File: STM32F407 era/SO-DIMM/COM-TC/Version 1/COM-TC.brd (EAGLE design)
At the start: 127 x 165.1 mm, 172 parts, among them J1 CON1, J2 CON1, J3 SO-DIMM-CPU, J4 FTDI_DEVICE, Q4 PMV20XNE, U1 IRF9332PBF, U10 SN65HVD232D, U11 MAX9926, U12 MCP6004-E/SL, U13 MCP6004-E/SL, U14 MCP6004-E/SL, U2 5V, U3 TPS54331D, U4 3,3V, U5 MAX9926, U6 MCP6004-E/SL, U7 LoPy, U8 GTL2000, X1 057-014-1

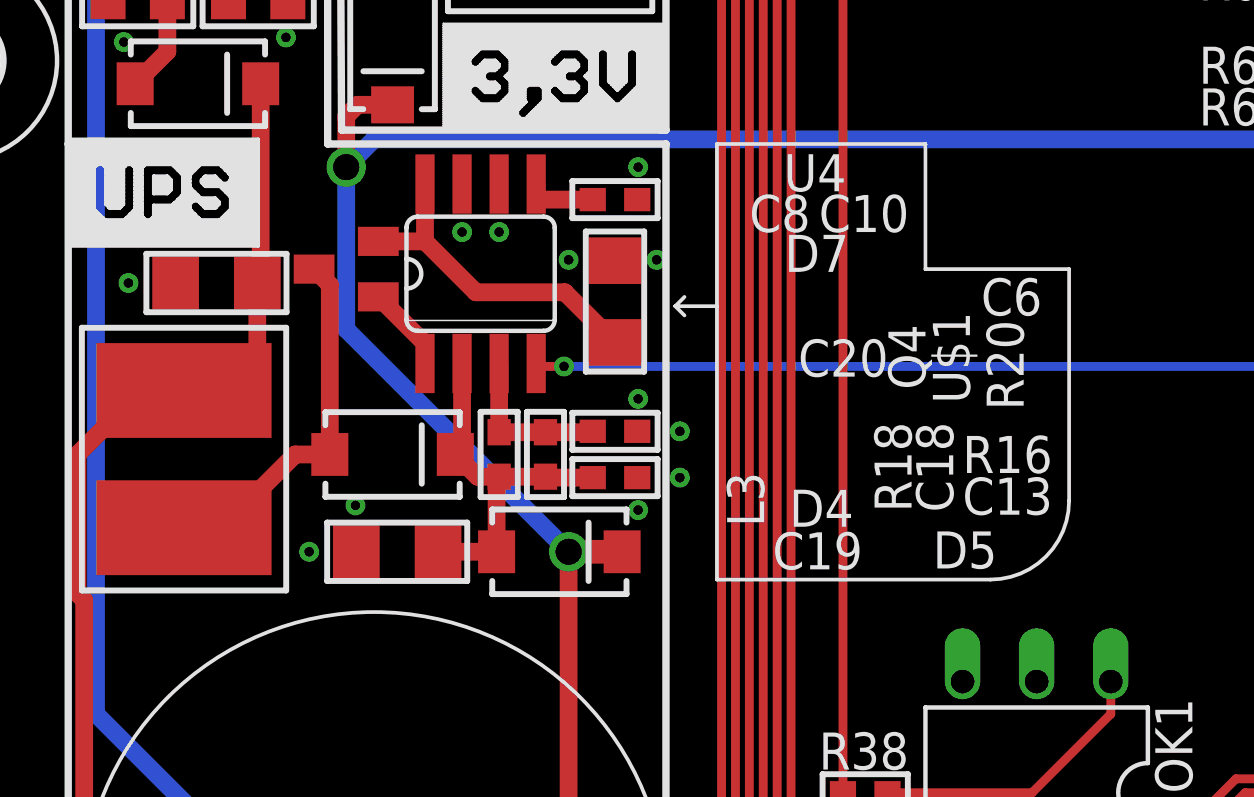
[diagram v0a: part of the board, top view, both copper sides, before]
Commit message: small error fixes
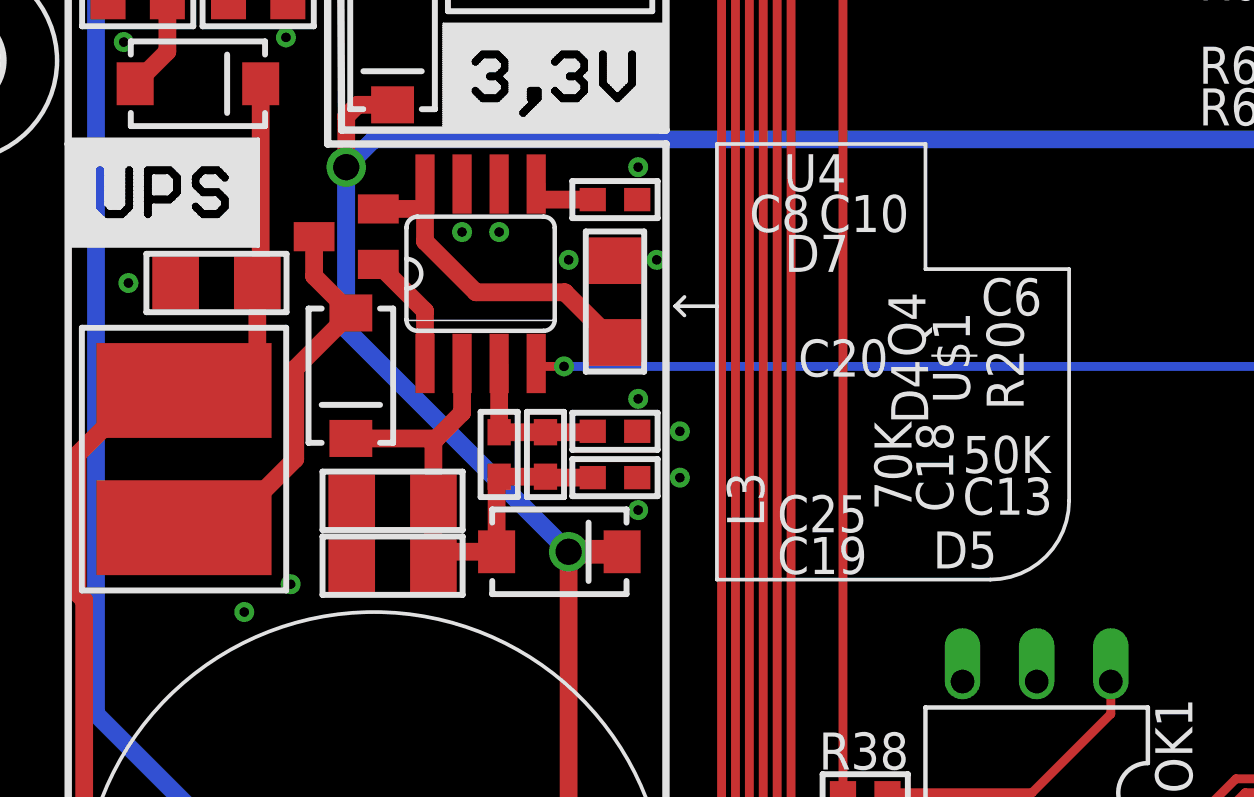
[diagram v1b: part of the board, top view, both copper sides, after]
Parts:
- added C25: 100u 6v3, microbuilder:1206
- C18: value 100n -> 47p
- C19: value 220u 6v3 -> 100u 6v3
- R20: value 10m -> 35m
- R69: value 3k24 -> 2k7
- moved D4 3.05 mm to (17.6, 76.2), turned to 270 degrees
- moved Q4 1.11 mm to (17.5, 81.0)
- moved C19 0.50 mm to (19.1, 69.7)
- renumbered R16 to 50K, R18 to 70K
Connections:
- net GND: now also C25.2
- net N$28: now also C25.1
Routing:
- net N$28: track 12.9 -> 18.5 mm
- net N$36: track 12.6 -> 15.0 mm
- net N$7: track 2.94 -> 4.06 mm
- net N$27: track 11.5 -> 12.4 mm

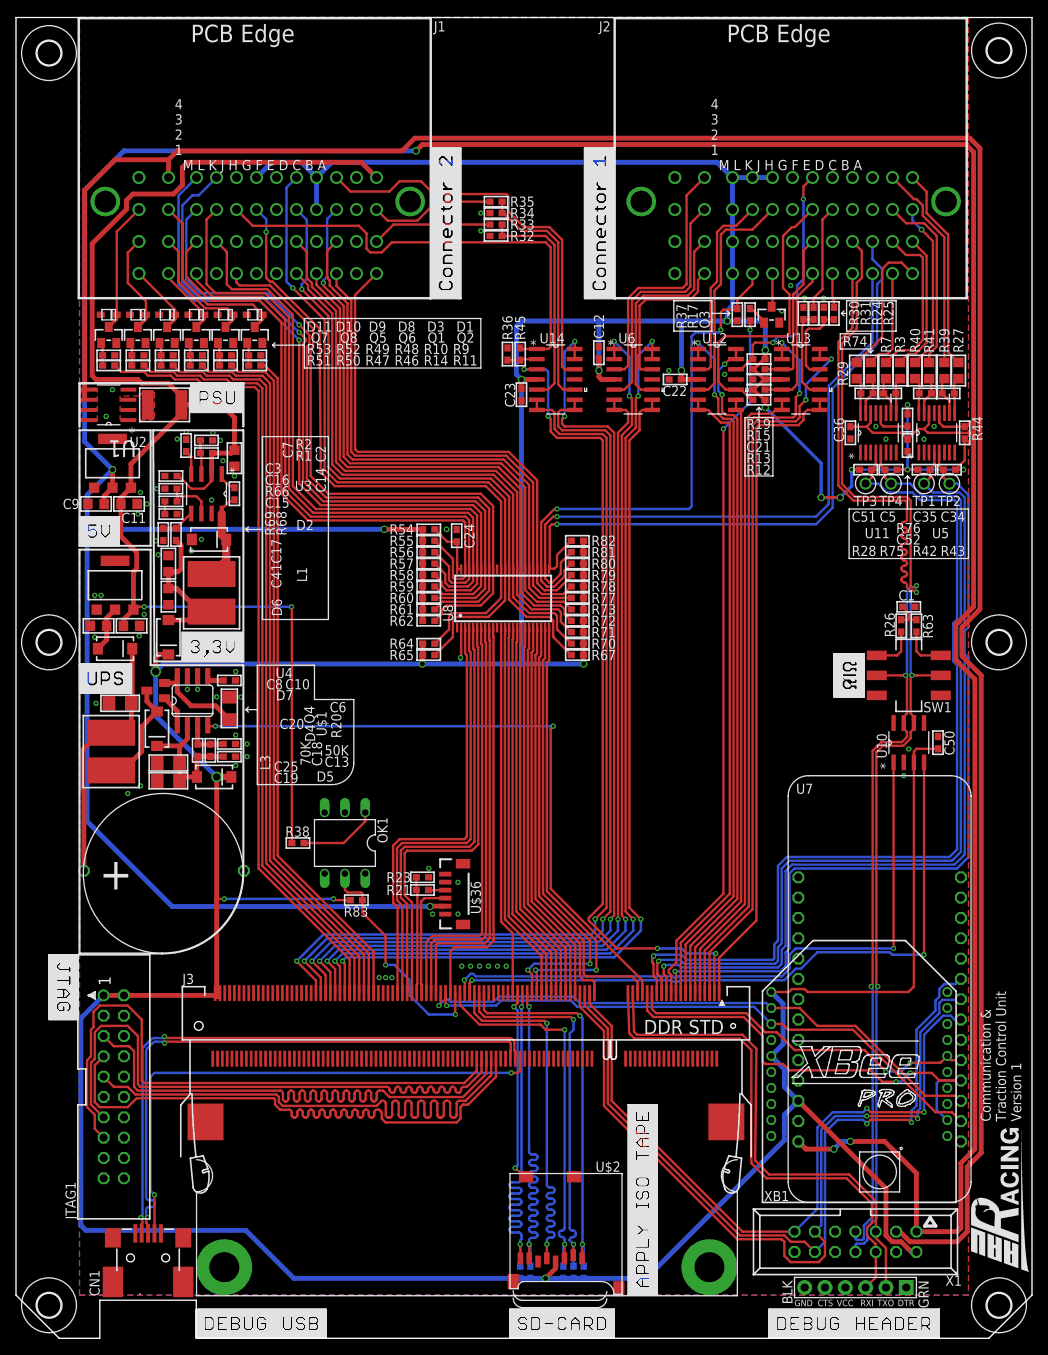
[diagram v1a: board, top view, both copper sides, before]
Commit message: error corrections
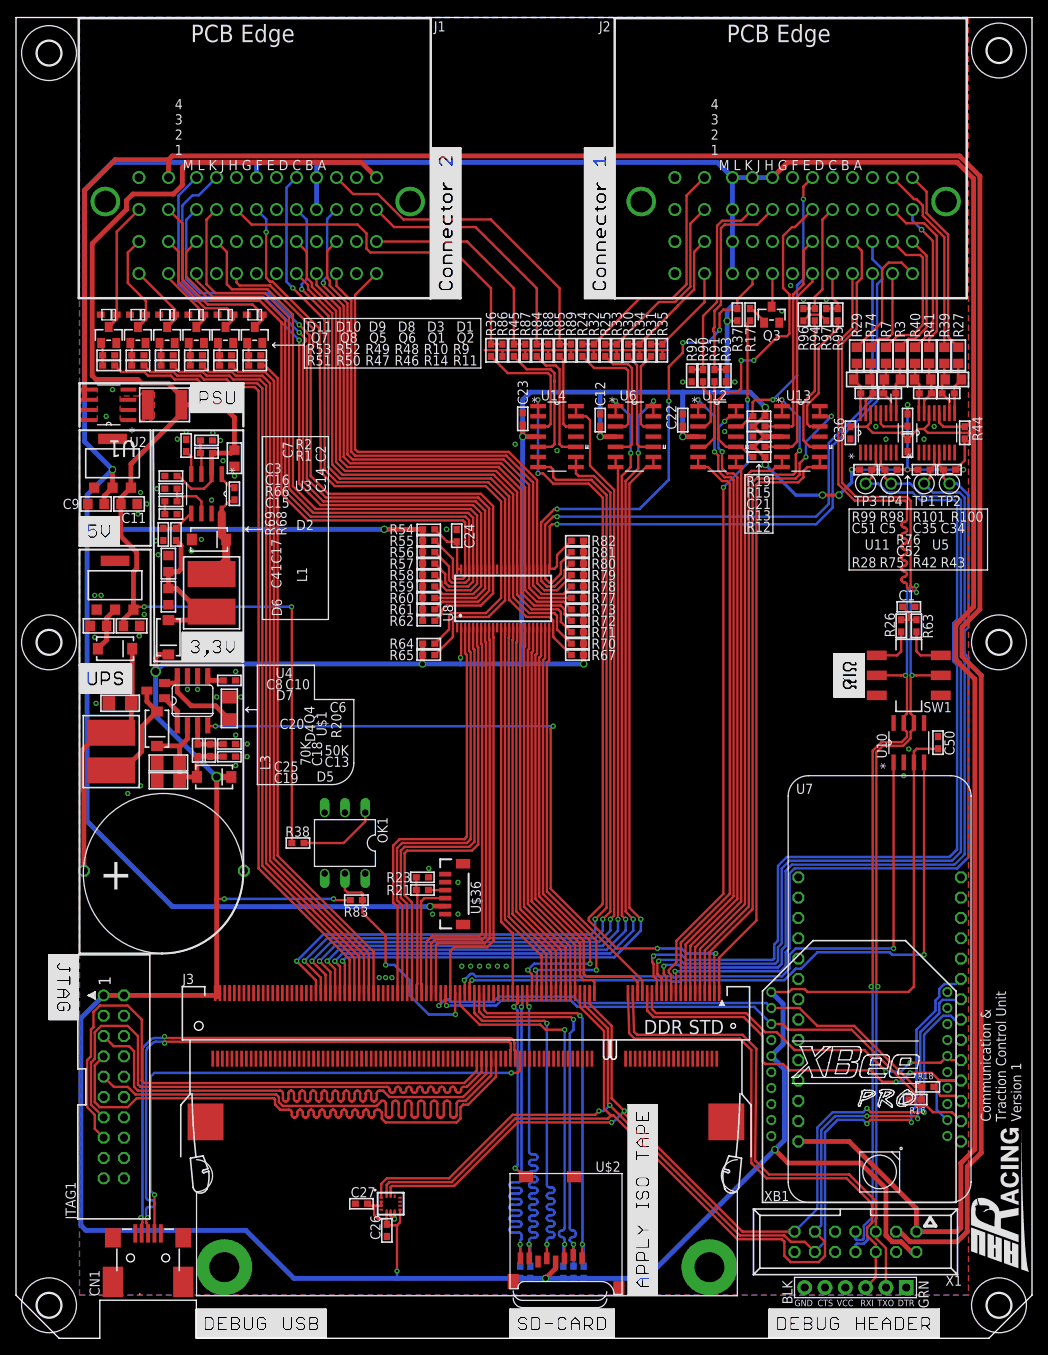
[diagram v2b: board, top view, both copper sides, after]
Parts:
- added C26, C27: 100n, microbuilder:_0603
- added R100, R101, R98, R99: 10k 0W5, microbuilder:_0805
- added R16, R86, R87, R88, R89, R92, R93, R96, R97: 976, microbuilder:_0603
- added R18, R84, R85, R90, R91, R94, R95: 499, microbuilder:_0603
- added U9: LSM6DS3, LSM6DS3:LGA14L_DOT_INDICATOR
- R24, R30, R36: value 976 -> 499
- R33, R35: value 499 -> 976
- moved R24 30.5 mm to (70.8, 123.5)
- moved R25 28.9 mm to (73.7, 123.5)
- moved R35 27.9 mm to (80.8, 123.5), turned to 270 degrees
- moved R34 24.8 mm to (77.9, 123.5), turned to 270 degrees
- moved R30 22.4 mm to (76.5, 123.5)
- moved R33 21.8 mm to (75.1, 123.5), turned to 270 degrees
- moved R31 20.8 mm to (79.4, 123.5)
- moved R32 18.8 mm to (72.2, 123.5), turned to 270 degrees
- moved C12 8.42 mm to (73.0, 114.8)
- moved U14 7.15 mm to (67.6, 112.7)
- moved U6 7.15 mm to (77.3, 112.7)
- moved R13 7.14 mm to (92.9, 111.4)
- moved C21 7.14 mm to (92.9, 112.7)
- moved R12 7.14 mm to (92.9, 110.2)
- moved R15 7.14 mm to (92.9, 114.0)
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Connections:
- removed net CURRENT1H: J2.E1, R25.1
- removed net CURRENT1L: R24.2, R25.2, U13.12
- removed net CURRENT2H: J2.E3, R31.1
- removed net CURRENT2L: R30.2, R31.2, U13.10
- removed net GSENSL: R32.2, R33.2, U14.5
- removed net VOUT: J3.3, U14.3
- removed net VOUTB: J1.H3, R45.2, U14.1
- removed net YAWL: R34.2, R35.2, U14.10
- new net CLUTCH-POT1: R31.2, U6.12
- new net CURRENT1: J2.E1, R95.1, R97.1
- new net CURRENT2: J2.E3, R94.1, R96.1
- new net GSENSL1: R25.2, U6.5
- new net GSENSL2: R91.2, U12.5
- new net GSENSL3: R95.2, U13.12
- new net N$34: R84.2, U14.10
- new net N$35: R18.2, U7.41
- new net N$38: R45.2, U14.5
- new net N$39: R36.2, U14.3
- new net STEERING-ANGLE: J1.H3, R36.1, R86.1
- new net STEERING-ANGLE1: R24.2, U6.3
- new net STEERING-ANGLE2: R90.2, U12.3
- new net STEERING-ANGLE3: R94.2, U13.10
- new net STEERING-ANGLEB: J3.3, U14.1, U14.2
- new net YAWL1: R30.2, U6.10
- net 3.3V: now also C26.1, C27.1, U9.2, U9.3, U9.5, U9.8; no longer J1.D3, J1.D4, J1.G4, J2.H4, J2.J4, J2.K1, J2.K2, J2.K3, J2.K4, U7.3,3V
- net 5.0V: now also J1.D3, J1.D4, J1.G4, J2.H4, J2.J4, J2.K1, J2.K2, J2.K3, J2.K4
- net CLUTCH-POT: now also R85.1, R89.1; no longer U14.12
- net GEARPOSAN: now also R91.1, R93.1; no longer U12.5
- net GND: now also C26.2, C27.2, R16.2, R32.2, R33.2, R34.2, R35.2, R86.2, R87.2, R88.2, R89.2, R92.2, R93.2, R96.2, R97.2, U9.12, U9.6, U9.7; no longer R24.1, R30.1, R32.1, R34.1, R36.1
- net GSENS: now also R45.1, R87.1; no longer R33.1
- net MISO: now also U9.1
- net MOSI: now also U9.14
- net N$11: now also R100.2
- net N$13: now also R85.2, U14.12; no longer R36.2, R45.1, U14.2
- net N$15: now also R101.1
- net N$16: now also R98.2
- net N$17: now also R101.2
- net N$18: now also R100.1
- net N$19: now also R99.1
- net N$25: now also R99.2
- net N$26: now also R98.1
- net SCK: now also U9.13
- net SPEED: now also R90.1, R92.1; no longer U12.3
- net TELE_RX: now also R16.1, R18.1; no longer U7.41
- net TRAVEL1: now also R25.1, R33.1; no longer U6.5
- net TRAVEL2: now also R24.1, R32.1; no longer U6.3
- net TRAVEL3: now also R30.1, R34.1; no longer U6.10
- net TRAVEL4: now also R31.1, R35.1; no longer U6.12
- net YAW: now also R84.1, R88.1; no longer R35.1
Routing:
- net VOUT: track 102.7 -> 0.00 mm, vias 4 -> 0
- net STEERING-ANGLEB: track 0.00 -> 96.8 mm, vias 0 -> 4
- net 3.3V: track 644.2 -> 560.6 mm, vias 20 -> 22
- net VOUTB: track 59.8 -> 0.00 mm
- net STEERING-ANGLE: track 0.00 -> 45.4 mm
- net GND: track 0.00 -> 34.7 mm, vias 62 -> 64
- net MISO: track 97.3 -> 131.7 mm, vias 2 -> 4
- net SCK: track 88.4 -> 122.7 mm, vias 2 -> 4
- net MOSI: track 100.4 -> 133.7 mm
- net YAWL: track 30.0 -> 0.00 mm
- net GSENSL: track 28.3 -> 0.00 mm
- net STEERING-ANGLE3: track 0.00 -> 17.9 mm
- net N$38: track 0.00 -> 17.2 mm
- net YAW: track 15.7 -> 32.5 mm
- net N$39: track 0.00 -> 16.2 mm
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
